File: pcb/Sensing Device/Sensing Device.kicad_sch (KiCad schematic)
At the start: 25 parts, among them J1 USB_C_Receptacle_PowerOnly_6P, SW1 SW_SPDT, SW2 SW_SPST, U2 MCP73831-2-OT, U3 TLV493D

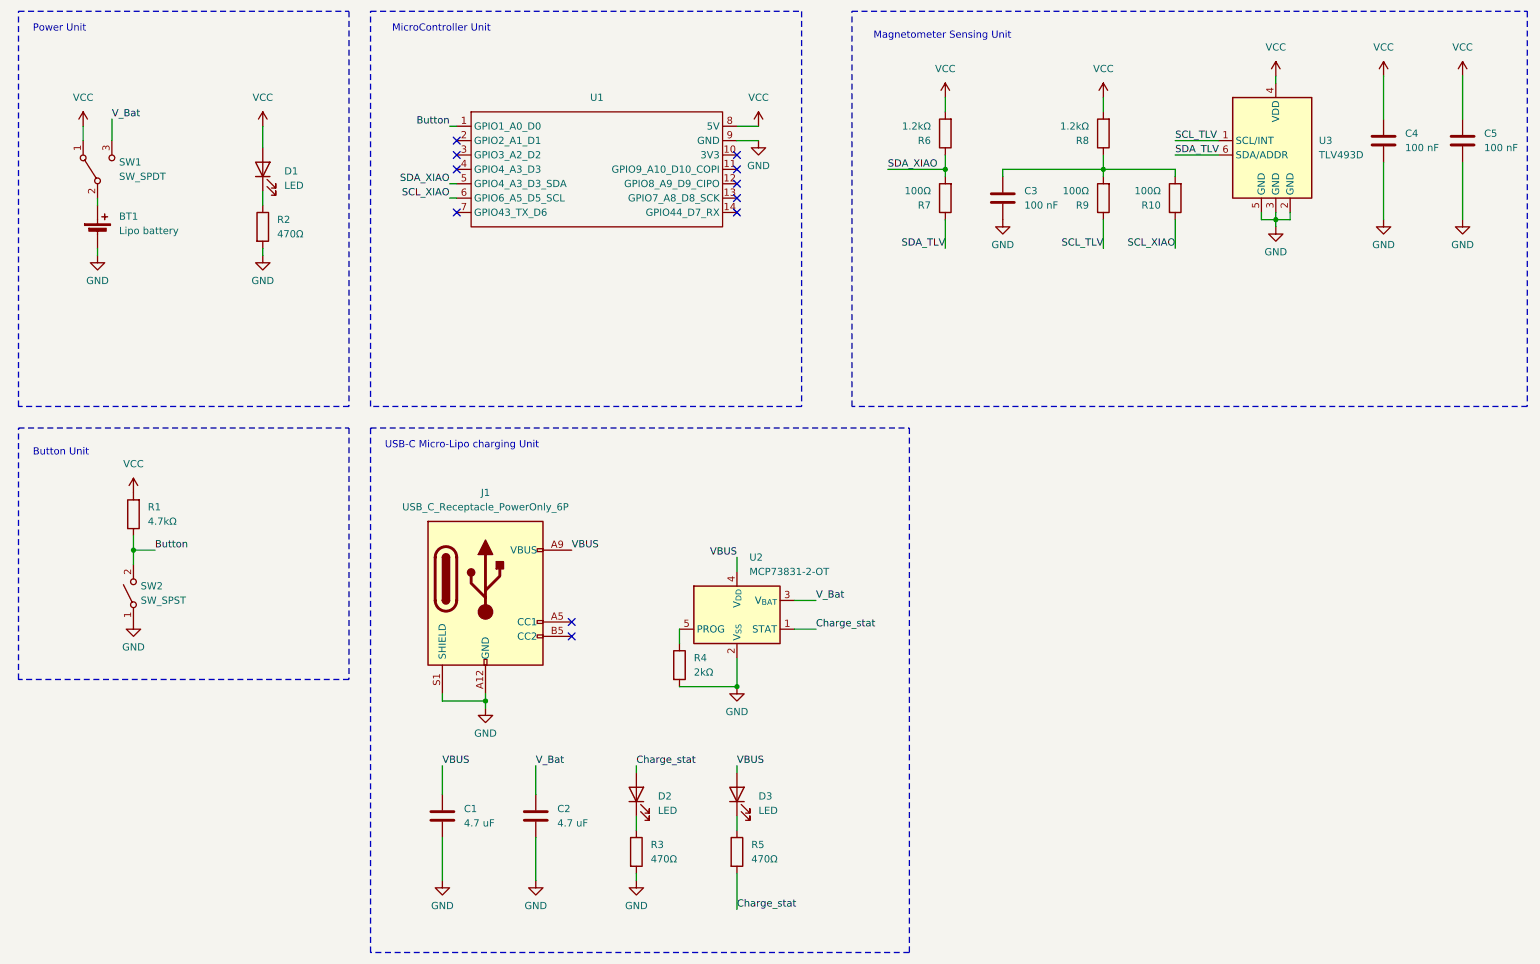
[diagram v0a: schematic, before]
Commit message: pcb update
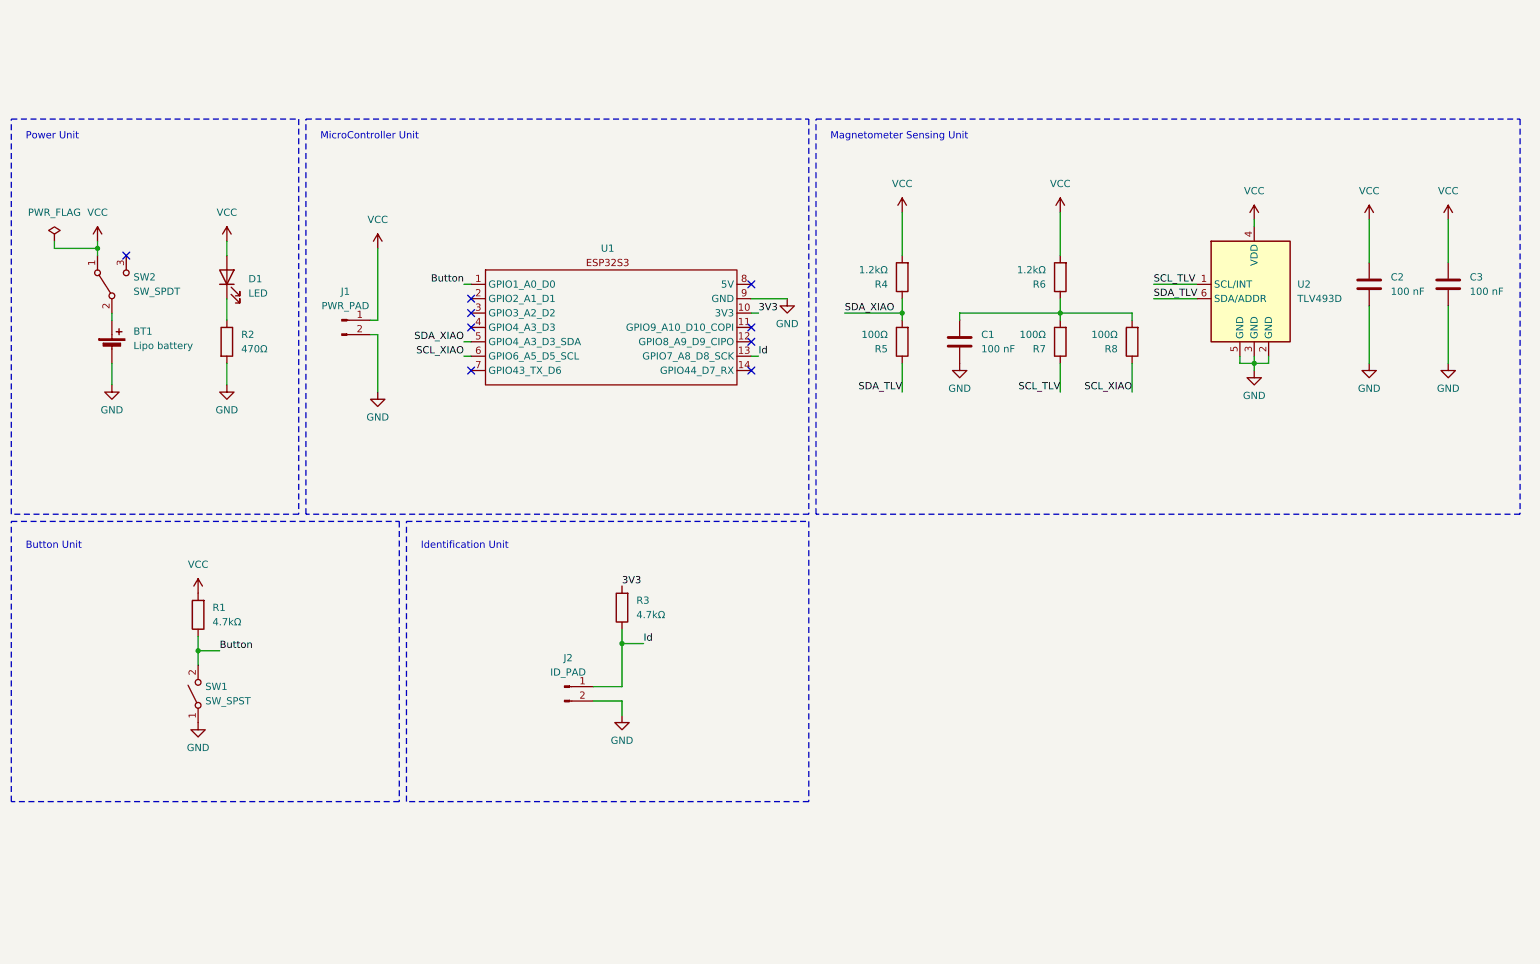
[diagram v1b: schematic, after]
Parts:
- removed C1, C2: 4.7 uF, symbol Device:C
- removed D2, D3: LED, symbol Device:LED
- removed J1: USB_C_Receptacle_PowerOnly_6P, symbol Connector:USB_C_Receptacle_PowerOnly_6P
- removed R4: 2kΩ, symbol Device:R
- removed R5: 470Ω, symbol Device:R
- removed U2: MCP73831-2-OT, Package_TO_SOT_SMD:SOT-23-5, symbol Battery_Management:MCP73831-2-OT
- added J1: PWR_PAD, Connector_JST:JST_NV_B02P-NV_1x02_P5.00mm_Vertical, symbol Connector:Conn_01x02_Pin
- added J2: ID_PAD, Screw_connector:40mm_rectangle_M3, symbol Connector:Conn_01x02_Pin
- BT1: footprint (none) -> Connector_JST:JST_ZE_SM02B-ZESS-TB_1x02-1MP_P1.50mm_Horizontal
- C1: renamed from C3; footprint (none) -> Capacitor_SMD:C_0805_2012Metric_Pad1.18x1.45mm_HandSolder
- C2: renamed from C4; footprint (none) -> Capacitor_SMD:C_0805_2012Metric_Pad1.18x1.45mm_HandSolder
- C3: renamed from C5; footprint (none) -> Capacitor_SMD:C_0805_2012Metric_Pad1.18x1.45mm_HandSolder
- D1: footprint (none) -> LED_THT:LED_D4.0mm
- R1, R2: footprint (none) -> Resistor_SMD:R_0805_2012Metric_Pad1.20x1.40mm_HandSolder
- R3: value 470Ω -> 4.7kΩ; footprint (none) -> Resistor_SMD:R_0805_2012Metric_Pad1.20x1.40mm_HandSolder
- R4: renamed from R6; footprint (none) -> Resistor_SMD:R_0805_2012Metric_Pad1.20x1.40mm_HandSolder
- R5: renamed from R7; footprint (none) -> Resistor_SMD:R_0805_2012Metric_Pad1.20x1.40mm_HandSolder
- R6: renamed from R8; footprint (none) -> Resistor_SMD:R_0805_2012Metric_Pad1.20x1.40mm_HandSolder
- R7: renamed from R9; footprint (none) -> Resistor_SMD:R_0805_2012Metric_Pad1.20x1.40mm_HandSolder
- R8: renamed from R10; footprint (none) -> Resistor_SMD:R_0805_2012Metric_Pad1.20x1.40mm_HandSolder
- SW1: renamed from SW2; footprint (none) -> Button_Switch_THT:SW_PUSH-12mm
- SW2: renamed from SW1; footprint (none) -> Button_Switch_THT:SWITCH_THT_SPDT_11MA1QS1
- U1: footprint (none) -> XIAO ESP32 THT:XIAO_ESP32_SENSE
- renumbered U3 to U2
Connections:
- net GND: now also J1.2 (Pin_2), J2.2 (Pin_2); no longer R3.2
- net VCC: now also J1.1 (Pin_1); no longer U1.8 (5V)
- net Id: now reaches R3.1
- net Id: now also U1.13 (GPIO7_A8_D8_SCK), J2.1 (Pin_1)
- net 3V3: now reaches U1.10 (3V3)
- net 3V3: now also R3.2
- net V_Bat: no longer names the net of SW2.3 (C)
- no-connect marks 11 -> 9
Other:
- note added: "Identification Unit"
- note removed: "USB-C Micro-Lipo charging Unit"
- moved on the sheet: BT1, C1, C2, C3, D1, R1, R2, R4, R5, R6, R7, R8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
